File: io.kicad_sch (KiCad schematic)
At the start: 23 parts, among them SW1 KMR221GLFS, SW2 KMR221GLFS, SW3 KMR221GLFS, SW4 KMR221GLFS, SW5 KMR221GLFS, SW6 KMR221GLFS, SW7 KMR221GLFS, U8 KMR241GLFS, U9 KMR241GLFS

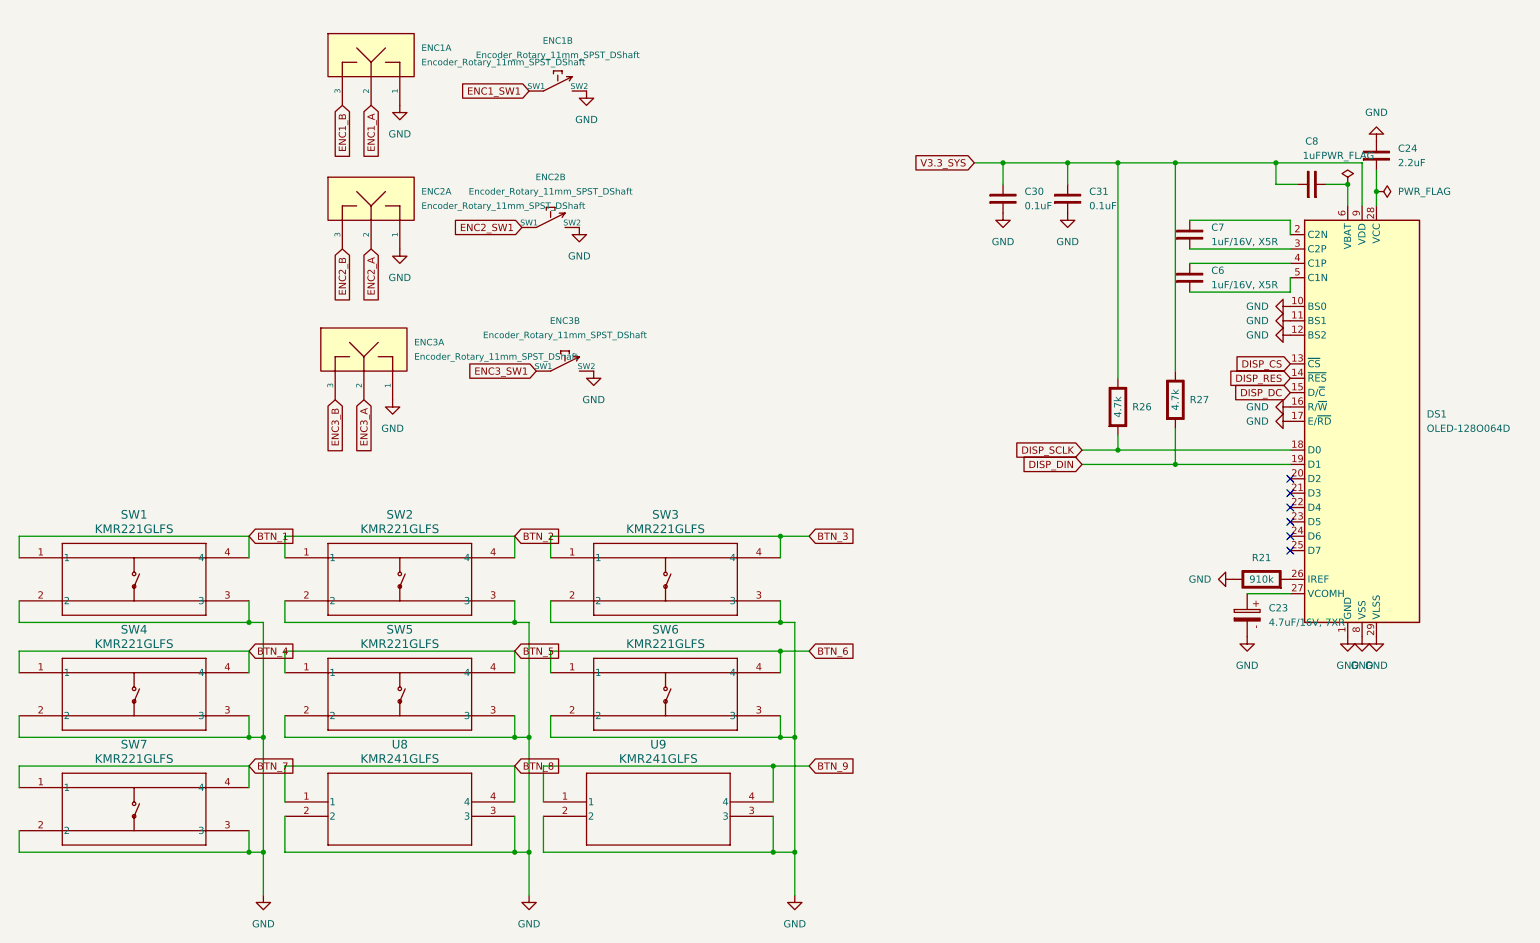
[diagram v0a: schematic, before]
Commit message: pcb / inital work
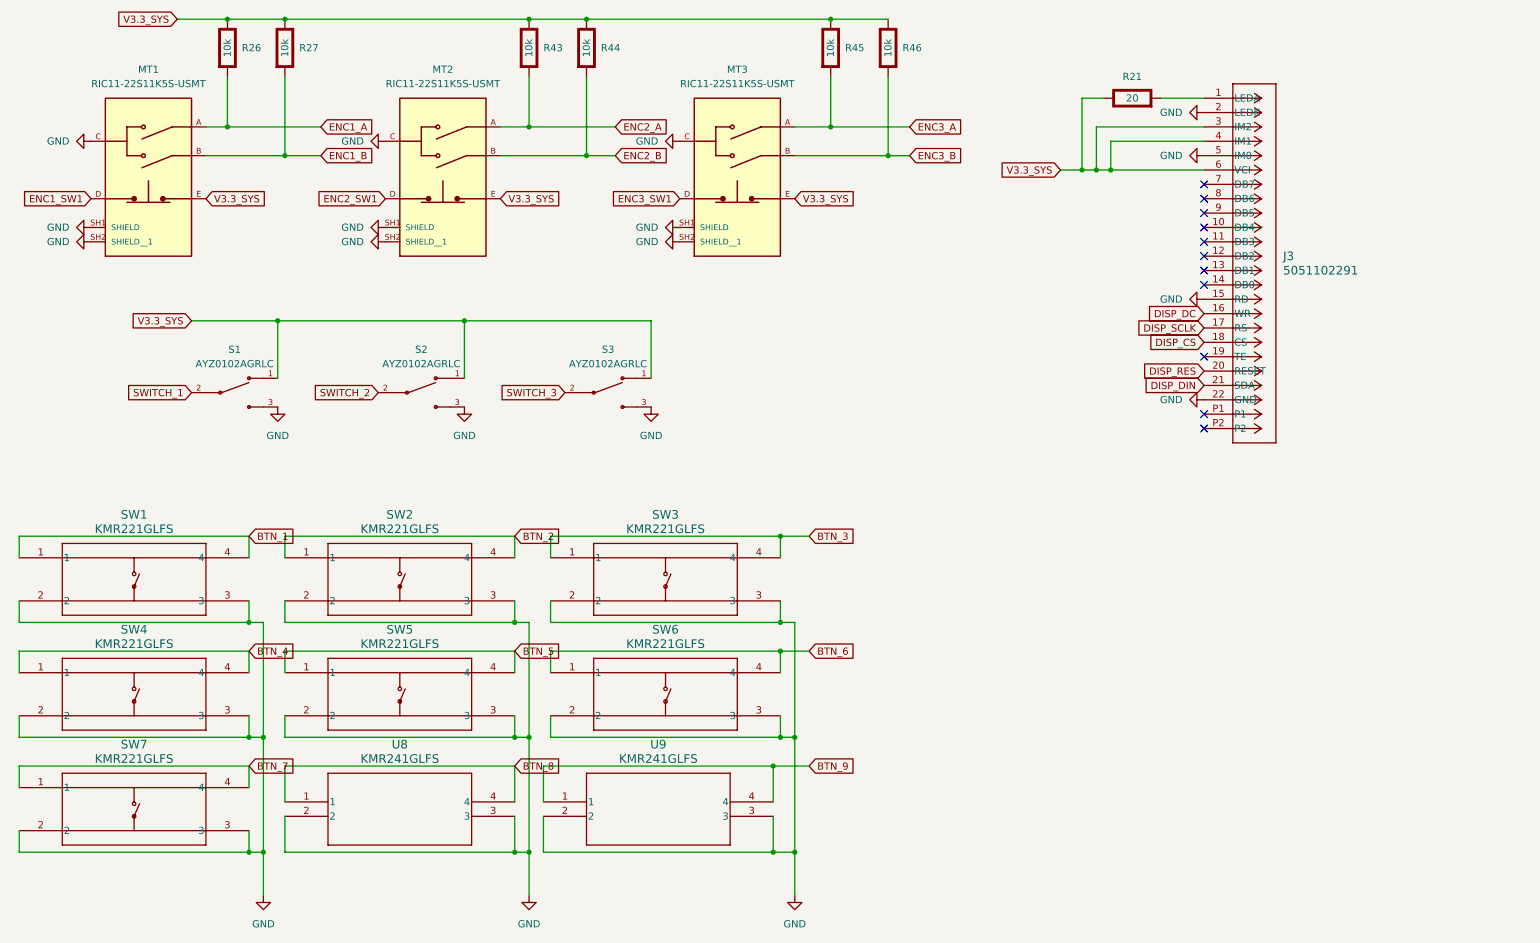
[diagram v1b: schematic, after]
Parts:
- removed C23: 4.7uF/16V, 7XR, Capacitor_THT:CP_Radial_D5.0mm_P2.50mm, symbol PCM_SL_Devices:Capacitor_PO
- removed C24: 2.2uF, Capacitor_THT:C_Disc_D3.0mm_W2.0mm_P2.50mm, symbol PCM_SL_Devices:Capacitor_NP
- removed C30, C31: 0.1uF, Capacitor_THT:C_Disc_D3.0mm_W2.0mm_P2.50mm, symbol PCM_SL_Devices:Capacitor_NP
- removed C6, C7: 1uF/16V, X5R, Capacitor_THT:C_Disc_D3.0mm_W2.0mm_P2.50mm, symbol PCM_SL_Devices:Capacitor_NP
- removed C8: 1uF, Capacitor_THT:C_Disc_D3.0mm_W2.0mm_P2.50mm, symbol PCM_SL_Devices:Capacitor_NP
- removed DS1: OLED-128O064D, Display:OLED-128O064D, symbol Display_Graphic:OLED-128O064D
- removed ENC1, ENC2, ENC3: Encoder_Rotary_11mm_SPST_DShaft, 4ms_Encoder:ENC_SPST_12mm, symbol PCM_4ms_Switch:Encoder_Rotary_11mm_SPST_DShaft
- added J3: 5051102291, CON_5051102291_MOL, symbol uwu:4421
- added MT1, MT2, MT3: RIC11-22S11K5S-USMT, uwu:XDCR_RIC11-22S11K5S-USMT, symbol uwu:RIC11-22S11K5S-USMT
- added R43, R44, R45, R46: 10k, Resistor_SMD:R_0603_1608Metric, symbol PCM_Elektuur:R
- added S1, S2, S3: AYZ0102AGRLC, uwu:SW_AYZ0102AGRLC, symbol uwu:AYZ0102AGRLC
- R21: value 910k -> 20; footprint (none) -> Resistor_SMD:R_0603_1608Metric
- R26, R27: value 4.7k -> 10k; footprint (none) -> Resistor_SMD:R_0603_1608Metric
- U8, U9: footprint SWITCH_241GLFS -> uwu:SWITCH_241GLFS
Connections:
- net DISP_CS: now also J3.18 (CS)
- net DISP_DC: now also J3.16 (WR)
- net DISP_DIN: now also J3.21 (SDA); no longer R27.2 (-)
- net DISP_RES: now also J3.20 (RESET)
- net DISP_SCLK: now also J3.17 (RS); no longer R26.2 (-)
- net ENC1_A: now also R26.2 (-), MT1.A
- net ENC1_B: now also R27.2 (-), MT1.B
- net ENC1_SW1: now also MT1.D
- net ENC2_A: now also MT2.A, R43.2 (-)
- net ENC2_B: now also MT2.B, R44.2 (-)
- net ENC2_SW1: now also MT2.D
- net ENC3_A: now also MT3.A, R45.2 (-)
- net ENC3_B: now also MT3.B, R46.2 (-)
- net ENC3_SW1: now also MT3.D
- net GND: now also J3.15 (RD), J3.2 (LEDK), J3.22 (GND), J3.5 (IM0), MT1.C, MT1.SH1 (SHIELD), MT1.SH2 (SHIELD__1), MT2.C, MT2.SH1 (SHIELD), MT2.SH2 (SHIELD__1), MT3.C, MT3.SH1 (SHIELD), MT3.SH2 (SHIELD__1), S1.3, S2.3, S3.3; no longer R21.1 (+)
- net V3.3_SYS: now also R21.1 (+), J3.3 (IM2), J3.4 (IM1), J3.6 (VCI), MT1.E, MT2.E, MT3.E, R43.1 (+), R44.1 (+), R45.1 (+), R46.1 (+), S1.1, S2.1, S3.1
- net at R21.2 (-): now also J3.1 (LEDA)
- new net SWITCH_1: S1.2
- new net SWITCH_2: S2.2
- new net SWITCH_3: S3.2
- no-connect marks 6 -> 11
